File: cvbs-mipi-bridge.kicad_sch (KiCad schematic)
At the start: 105 parts, among them IC1 ADV7280BCPZ-M, IC2 TLV70018, IC4 SN74AUP1G17DCKR, IC5 SN74AUP1G17DCKR, J1 WE_68715014522, J2 61300211121, J7 61300211121, Q1 BSS138APW, Q2 BSS138APW, Q3 BSS138APW, Q4 BSS138APW, Y1 ABM8G-28.63636MHZ-18-D2Y-T

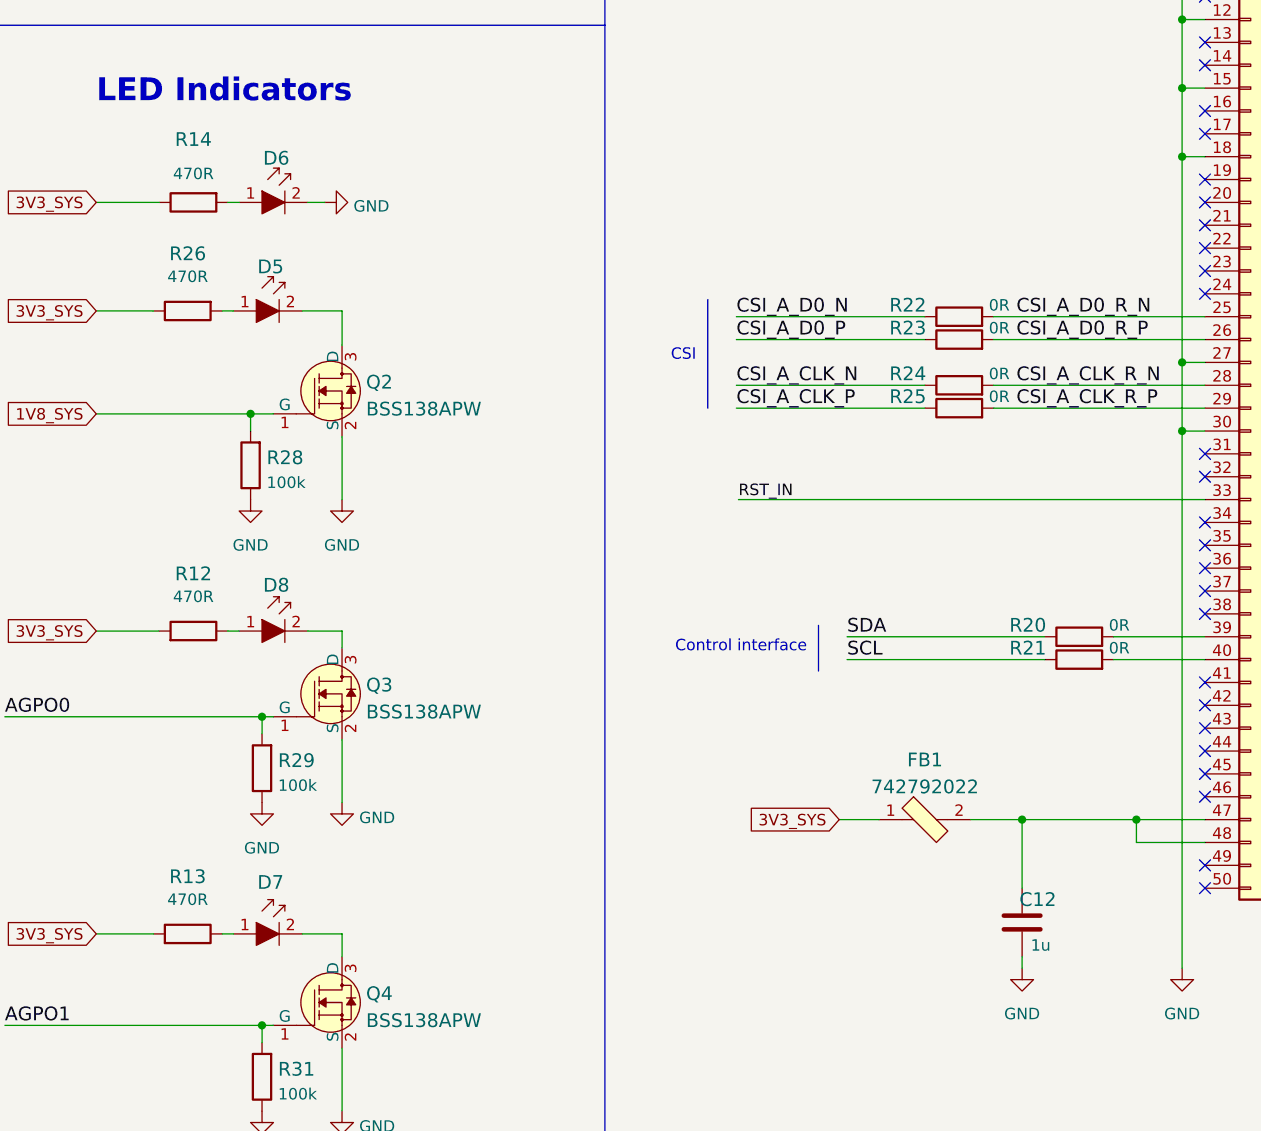
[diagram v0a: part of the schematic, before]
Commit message: Cleanup
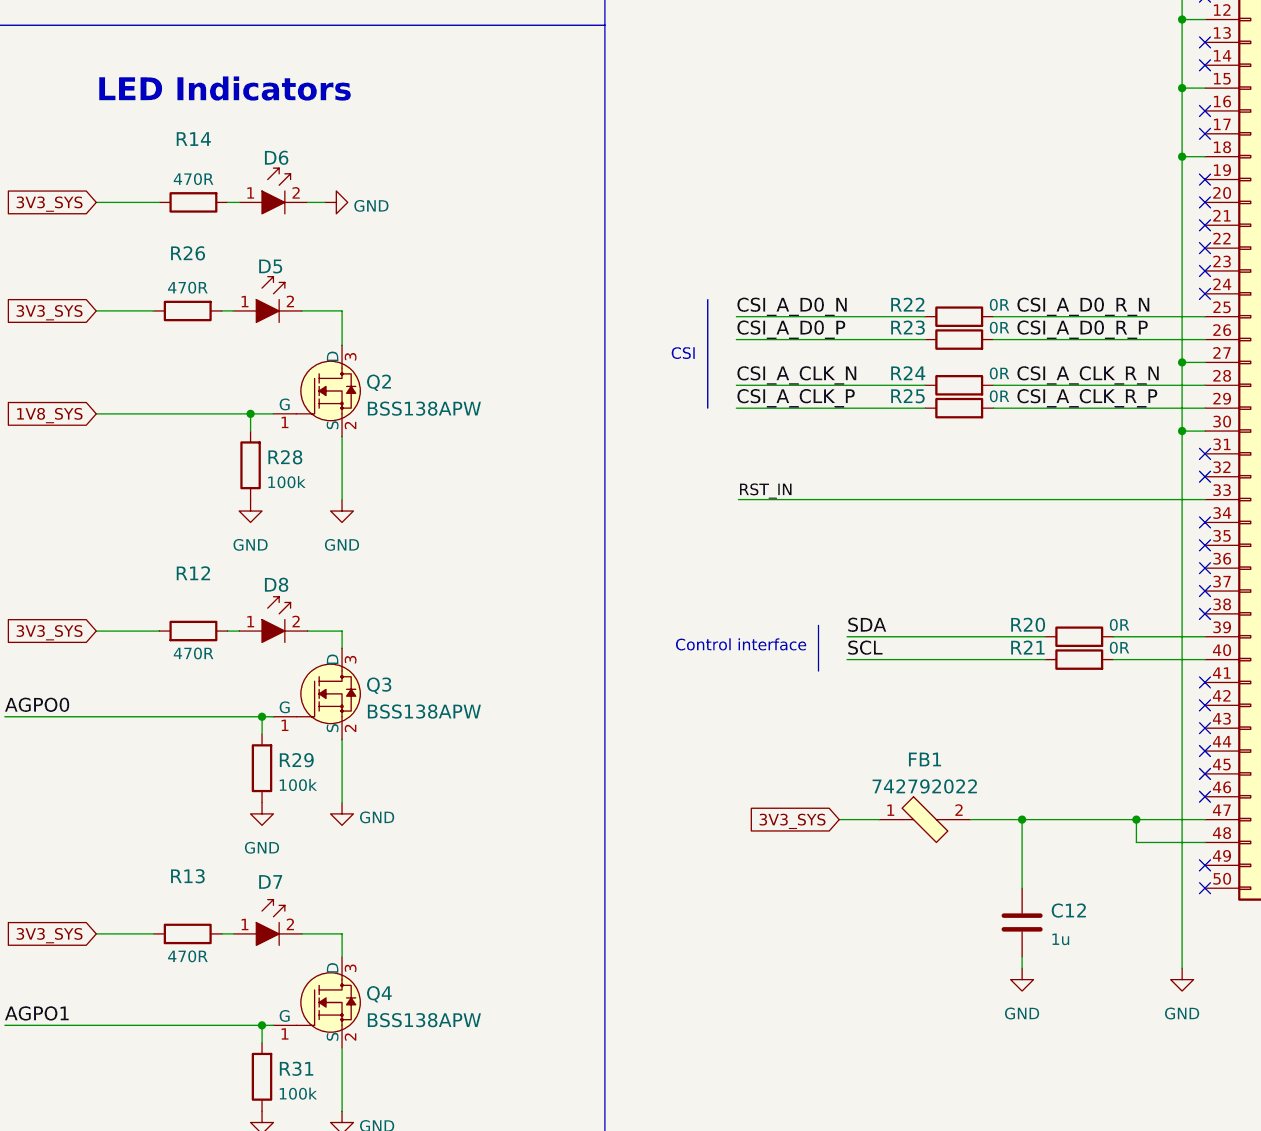
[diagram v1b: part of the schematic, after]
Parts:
- removed C12: C_1u_0603, antmicro-cvbs-mipi-bridge-footprints:0603-cap, symbol antmicro-cvbs-mipi-bridge:C_1u_0603
- added C12: C_1u_0603, cvbs-mipi-bridge-footprints:0603-cap, symbol cvbs-mipi-bridge:C_1u_0603
- AIN1, AIN2, AIN3, AIN4: footprint antmicro-cvbs-mipi-bridge-footprints:PJRAN1X1U01X -> cvbs-mipi-bridge-footprints:PJRAN1X1U01X; symbol antmicro-cvbs-mipi-bridge:PJRAN1X1U01X -> cvbs-mipi-bridge:PJRAN1X1U01X
- C1, C10, C13, C14, C16, C17, C2, C20, C21, C24, C26, C3, C4, C5, C6, C7: footprint antmicro-cvbs-mipi-bridge-footprints:0402-cap -> cvbs-mipi-bridge-footprints:0402-cap; symbol antmicro-cvbs-mipi-bridge:C_100n_0402 -> cvbs-mipi-bridge:C_100n_0402
- C11, C15, C18, C19: footprint antmicro-cvbs-mipi-bridge-footprints:0402-cap -> cvbs-mipi-bridge-footprints:0402-cap; symbol antmicro-cvbs-mipi-bridge:C_10n_0402 -> cvbs-mipi-bridge:C_10n_0402
- C22, C23: footprint antmicro-cvbs-mipi-bridge-footprints:0402-cap -> cvbs-mipi-bridge-footprints:0402-cap; symbol antmicro-cvbs-mipi-bridge:C_10p_0402 -> cvbs-mipi-bridge:C_10p_0402
- C27, C28, C8, C9: footprint antmicro-cvbs-mipi-bridge-footprints:0402-cap -> cvbs-mipi-bridge-footprints:0402-cap; symbol antmicro-cvbs-mipi-bridge:C_1u_0402 -> cvbs-mipi-bridge:C_1u_0402
- D1, D2, D3, D4: footprint antmicro-cvbs-mipi-bridge-footprints:SOT-23-3 -> cvbs-mipi-bridge-footprints:SOT-23-3; symbol antmicro-cvbs-mipi-bridge:PESD1CAN_215 -> cvbs-mipi-bridge:PESD1CAN_215
- D5, D6, D7, D8: footprint antmicro-cvbs-mipi-bridge-footprints:LED_0603 -> cvbs-mipi-bridge-footprints:LED_0603; symbol antmicro-cvbs-mipi-bridge:KP-1608ZGC -> cvbs-mipi-bridge:KP-1608ZGC
- FB1, FB3, FB4, FB5: footprint antmicro-cvbs-mipi-bridge-footprints:0805-res -> cvbs-mipi-bridge-footprints:0805-res; symbol antmicro-cvbs-mipi-bridge:742792022 -> cvbs-mipi-bridge:742792022
- IC1: footprint antmicro-cvbs-mipi-bridge-footprints:LFCSP-32-1EP-5x5mm -> cvbs-mipi-bridge-footprints:LFCSP-32-1EP-5x5mm; symbol antmicro-cvbs-mipi-bridge:ADV7280BCPZ-M -> cvbs-mipi-bridge:ADV7280BCPZ-M
- IC2: footprint antmicro-cvbs-mipi-bridge-footprints:SC-70-5 -> cvbs-mipi-bridge-footprints:SC-70-5; symbol antmicro-cvbs-mipi-bridge:TLV70018 -> cvbs-mipi-bridge:TLV70018
- IC4, IC5: footprint antmicro-cvbs-mipi-bridge-footprints:SOT-753 -> cvbs-mipi-bridge-footprints:SOT-753; symbol antmicro-cvbs-mipi-bridge:SN74AUP1G17DCKR -> cvbs-mipi-bridge:SN74AUP1G17DCKR
- J1: footprint antmicro-cvbs-mipi-bridge-footprints:WE_68715014522 -> cvbs-mipi-bridge-footprints:WE_68715014522; symbol antmicro-cvbs-mipi-bridge:WE_68715014522 -> cvbs-mipi-bridge:WE_68715014522
- J2, J7: footprint antmicro-cvbs-mipi-bridge-footprints:PinHeader_1x2_P2.54_Drill0.9mm -> cvbs-mipi-bridge-footprints:PinHeader_1x2_P2.54_Drill0.9mm; symbol antmicro-cvbs-mipi-bridge:61300211121 -> cvbs-mipi-bridge:61300211121
- MP1, MP2, MP3, MP4: footprint antmicro-cvbs-mipi-bridge-footprints:9774030243R -> cvbs-mipi-bridge-footprints:9774030243R; symbol antmicro-cvbs-mipi-bridge:9774030243R -> cvbs-mipi-bridge:9774030243R
- N1: footprint antmicro-cvbs-mipi-bridge-footprints:antmicro-logo_scaled_20mm -> cvbs-mipi-bridge-footprints:antmicro-logo_scaled_20mm; symbol antmicro-cvbs-mipi-bridge:antmicro_logo -> cvbs-mipi-bridge:antmicro_logo
- N2: footprint antmicro-cvbs-mipi-bridge-footprints:oshw-logo -> cvbs-mipi-bridge-footprints:oshw-logo; symbol antmicro-cvbs-mipi-bridge:oshw_logo -> cvbs-mipi-bridge:oshw_logo
- Q1, Q2, Q3, Q4: footprint antmicro-cvbs-mipi-bridge-footprints:SC70-3 -> cvbs-mipi-bridge-footprints:SC70-3; symbol antmicro-cvbs-mipi-bridge:BSS138APW -> cvbs-mipi-bridge:BSS138APW
- R1, R10, R4, R8: footprint antmicro-cvbs-mipi-bridge-footprints:0603-res -> cvbs-mipi-bridge-footprints:0603-res; symbol antmicro-cvbs-mipi-bridge:R_24R_0603 -> cvbs-mipi-bridge:R_24R_0603
- R11, R3, R5, R9: footprint antmicro-cvbs-mipi-bridge-footprints:0402-res -> cvbs-mipi-bridge-footprints:0402-res; symbol antmicro-cvbs-mipi-bridge:R_51R_0402 -> cvbs-mipi-bridge:R_51R_0402
- R12, R13, R14, R26: footprint antmicro-cvbs-mipi-bridge-footprints:0402-res -> cvbs-mipi-bridge-footprints:0402-res; symbol antmicro-cvbs-mipi-bridge:R_470R_0402 -> cvbs-mipi-bridge:R_470R_0402
- R15: footprint antmicro-cvbs-mipi-bridge-footprints:0402-res -> cvbs-mipi-bridge-footprints:0402-res; symbol antmicro-cvbs-mipi-bridge:R_22k_0402 -> cvbs-mipi-bridge:R_22k_0402
- R16: footprint antmicro-cvbs-mipi-bridge-footprints:0402-res -> cvbs-mipi-bridge-footprints:0402-res; symbol antmicro-cvbs-mipi-bridge:R_1M0_0402 -> cvbs-mipi-bridge:R_1M0_0402
- R17, R18, R19, R27, R28, R29, R31: footprint antmicro-cvbs-mipi-bridge-footprints:0402-res -> cvbs-mipi-bridge-footprints:0402-res; symbol antmicro-cvbs-mipi-bridge:R_100k_0402 -> cvbs-mipi-bridge:R_100k_0402
- R2: footprint antmicro-cvbs-mipi-bridge-footprints:0402-res -> cvbs-mipi-bridge-footprints:0402-res; symbol antmicro-cvbs-mipi-bridge:R_1k_0402 -> cvbs-mipi-bridge:R_1k_0402
- R20, R21, R22, R23, R24, R25, R30: footprint antmicro-cvbs-mipi-bridge-footprints:0402-res -> cvbs-mipi-bridge-footprints:0402-res; symbol antmicro-cvbs-mipi-bridge:R_0R_0402 -> cvbs-mipi-bridge:R_0R_0402
- R6, R7: footprint antmicro-cvbs-mipi-bridge-footprints:0402-res -> cvbs-mipi-bridge-footprints:0402-res; symbol antmicro-cvbs-mipi-bridge:R_4k7_0402 -> cvbs-mipi-bridge:R_4k7_0402
- S1: footprint antmicro-cvbs-mipi-bridge-footprints:SW_SPST_4.2x2.8 -> cvbs-mipi-bridge-footprints:SW_SPST_4.2x2.8; symbol antmicro-cvbs-mipi-bridge:KMR2 -> cvbs-mipi-bridge:KMR2
- TP1, TP10, TP11, TP12, TP13, TP2, TP3, TP5, TP6, TP7, TP8, TP9: footprint antmicro-cvbs-mipi-bridge-footprints:TP-R-1.5 -> cvbs-mipi-bridge-footprints:TP-R-1.5; symbol antmicro-cvbs-mipi-bridge:TP -> cvbs-mipi-bridge:TP
- Y1: footprint antmicro-cvbs-mipi-bridge-footprints:KX-7 -> cvbs-mipi-bridge-footprints:KX-7; symbol antmicro-cvbs-mipi-bridge:ABM8G-28.63636MHZ-18-D2Y-T -> cvbs-mipi-bridge:ABM8G-28.63636MHZ-18-D2Y-T
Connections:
- net GND: now also C12.2
- net at FB1.2, J1.47 (Pin_47), J1.48 (Pin_48): now also C12.1
